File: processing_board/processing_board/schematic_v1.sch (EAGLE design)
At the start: 20 parts, among them Q1 BSS138, Q2 BSS138

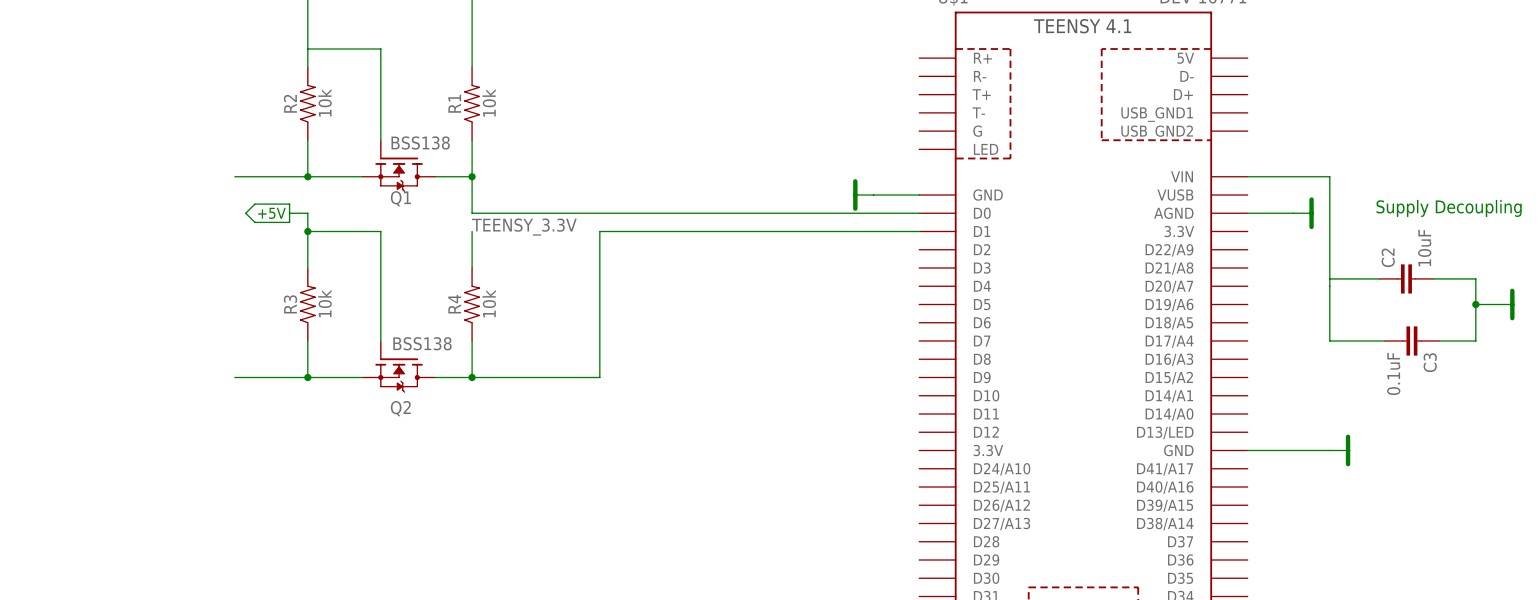
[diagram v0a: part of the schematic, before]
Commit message: modified shcematic and board
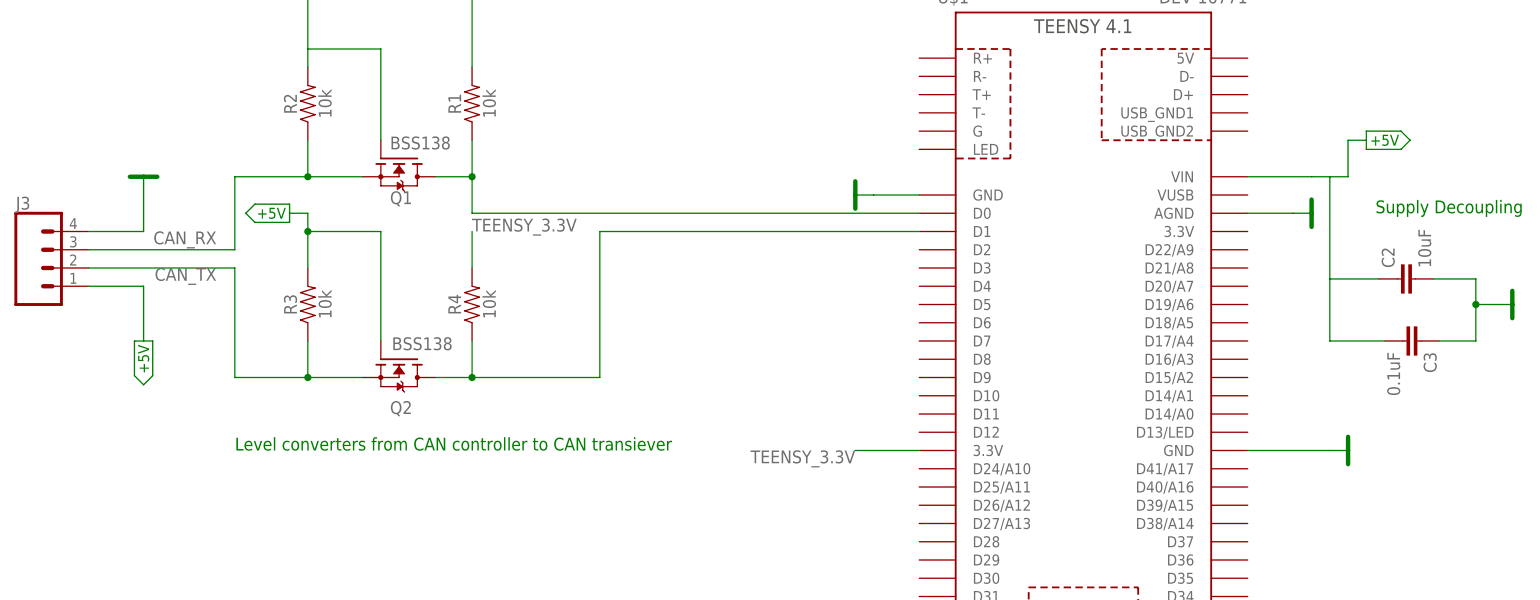
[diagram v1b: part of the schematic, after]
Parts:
- added J3: (no value), SparkFun-Connectors:CONN_04PTH
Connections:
- removed net N$11: Q2.S, R3.1
- removed net N$2: Q1.S, R2.1
- removed net VDD: C2.1, C3.2, U$1.VIN
- new net CAN_RX: J3.3, Q1.S, R2.1
- new net CAN_TX: J3.2, Q2.S, R3.1
- net +5V: now also C2.1, C3.2, J3.1, U$1.VIN
- net GND: now also J3.4
- net TEENSY_3.3V: now also U$1.3.3V
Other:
- note added: "Level converters from CAN controller to CAN transiever"
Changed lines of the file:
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@@
 <part name="PWR6" library="supply" deviceset="+5V" device=""/>
 <part name="PWR7" library="supply" deviceset="+5V" device=""/>
+<part name="PWR8" library="supply" deviceset="+5V" device=""/>
+<part name="J3" library="SparkFun-Connectors" deviceset="CONN_04" device="PTH"/>
+<part name="GND8" library="supply" deviceset="GND" device=""/>
+<part name="PWR9" library="supply" deviceset="+5V" device=""/>
 </parts>
 <sheets>
@@
 <plain>
 <text x="62.23" y="63.5" size="1.778" layer="91">Supply Decoupling</text>
+<text x="-96.52" y="30.48" size="1.778" layer="91">Level converters from CAN controller to CAN transiever</text>
 </plain>
 <instances>
@@
 <instance part="PWR6" gate="G$1" x="-86.36" y="93.98" smashed="yes"/>
 <instance part="PWR7" gate="G$1" x="-88.9" y="63.5" smashed="yes" rot="R90"/>
+<instance part="PWR8" gate="G$1" x="60.96" y="73.66" smashed="yes" rot="R270"/>
+<instance part="J3" gate="J1" x="-121.92" y="55.88" smashed="yes">
+<attribute name="VALUE" x="-127" y="48.514" size="1.778" layer="96" font="vector"/>
+<attribute name="NAME" x="-127" y="64.008" size="1.778" layer="95" font="vector"/>
+</instance>
+<instance part="GND8" gate="VR1" x="-109.22" y="68.58" smashed="yes" rot="R180"/>
+<instance part="PWR9" gate="G$1" x="-109.22" y="45.72" smashed="yes" rot="R180"/>
 </instances>
 <busses>
 </busses>
 <nets>
-<net name="VDD" class="0">
-<segment>
-<pinref part="C3" gate="G$1" pin="2"/>
-<wire x1="55.88" y1="54.356" x2="55.88" y2="53.34" width="0.1524" layer="91"/>
-<wire x1="55.88" y1="53.34" x2="55.88" y2="45.72" width="0.1524" layer="91"/>
-<wire x1="63.5" y1="45.72" x2="55.88" y2="45.72" width="0.1524" layer="91"/>
-<pinref part="C2" gate="G$1" pin="1"/>
-<wire x1="62.738" y1="54.356" x2="55.88" y2="54.356" width="0.1524" layer="91"/>
-<pinref part="U$1" gate="G$1" pin="VIN"/>
-<wire x1="44.45" y1="68.58" x2="55.88" y2="68.58" width="0.1524" layer="91"/>
-<wire x1="55.88" y1="68.58" x2="55.88" y2="54.356" width="0.1524" layer="91"/>
-</segment>
-</net>
 <net name="GND" class="0">
 <segment>
@@
 <wire x1="200.66" y1="45.72" x2="200.66" y2="48.26" width="0.1524" layer="91"/>
 </segment>
+<segment>
+<pinref part="J3" gate="J1" pin="4"/>
+<wire x1="-116.84" y1="60.96" x2="-109.22" y2="60.96" width="0.1524" layer="91"/>
+<wire x1="-109.22" y1="60.96" x2="-109.22" y2="66.04" width="0.1524" layer="91"/>
+<pinref part="GND8" gate="VR1" pin="GND"/>
+</segment>
 </net>
 <net name="+15V" class="0">
@@
 <wire x1="-88.9" y1="63.5" x2="-86.36" y2="63.5" width="0.1524" layer="91"/>
 </segment>
+<segment>
+<pinref part="PWR8" gate="G$1" pin="+5V"/>
+<wire x1="60.96" y1="73.66" x2="58.42" y2="73.66" width="0.1524" layer="91"/>
+<wire x1="58.42" y1="73.66" x2="58.42" y2="68.58" width="0.1524" layer="91"/>
+<pinref part="C3" gate="G$1" pin="2"/>
+<wire x1="55.88" y1="54.356" x2="55.88" y2="45.72" width="0.1524" layer="91"/>
+<wire x1="63.5" y1="45.72" x2="55.88" y2="45.72" width="0.1524" layer="91"/>
+<pinref part="C2" gate="G$1" pin="1"/>
+<wire x1="62.738" y1="54.356" x2="55.88" y2="54.356" width="0.1524" layer="91"/>
+<pinref part="U$1" gate="G$1" pin="VIN"/>
+<wire x1="44.45" y1="68.58" x2="53.34" y2="68.58" width="0.1524" layer="91"/>
+<wire x1="53.34" y1="68.58" x2="55.88" y2="68.58" width="0.1524" layer="91"/>
+<wire x1="55.88" y1="68.58" x2="55.88" y2="54.356" width="0.1524" layer="91"/>
+<wire x1="58.42" y1="68.58" x2="55.88" y2="68.58" width="0.1524" layer="91"/>
+</segment>
+<segment>
+<pinref part="J3" gate="J1" pin="1"/>
+<wire x1="-116.84" y1="53.34" x2="-109.22" y2="53.34" width="0.1524" layer="91"/>
+<wire x1="-109.22" y1="53.34" x2="-109.22" y2="45.72" width="0.1524" layer="91"/>
+<pinref part="PWR9" gate="G$1" pin="+5V"/>
+</segment>
 </net>
 <net name="+3.3V" class="0">
@@
 </segment>
 </net>
-<net name="N$2" class="0">
+<net name="CAN_RX" class="0">
 <segment>
 <pinref part="R2" gate="G$1" pin="1"/>
@@
 <wire x1="-86.36" y1="68.58" x2="-96.52" y2="68.58" width="0.1524" layer="91"/>
 <junction x="-86.36" y="68.58"/>
+<pinref part="J3" gate="J1" pin="3"/>
+<wire x1="-116.84" y1="58.42" x2="-96.52" y2="58.42" width="0.1524" layer="91"/>
+<wire x1="-96.52" y1="58.42" x2="-96.52" y2="68.58" width="0.1524" layer="91"/>
+<label x="-99.06" y="60.96" size="1.778" layer="95" rot="R180"/>
 </segment>
 </net>
@@
 <label x="-63.5" y="60.96" size="1.778" layer="95"/>
 </segment>
-</net>
-<net name="N$11" class="0">
+<segment>
+<pinref part="U$1" gate="G$1" pin="3.3V"/>
+<wire x1="-1.27" y1="30.48" x2="-10.16" y2="30.48" width="0.1524" layer="91"/>
+<label x="-10.16" y="30.48" size="1.778" layer="95" rot="R180"/>
+</segment>
+</net>
+<net name="CAN_TX" class="0">
 <segment>
 <pinref part="R3" gate="G$1" pin="1"/>
@@
 <wire x1="-86.36" y1="40.64" x2="-96.52" y2="40.64" width="0.1524" layer="91"/>
 <junction x="-86.36" y="40.64"/>
-</segment>
-</net>
+<wire x1="-96.52" y1="40.64" x2="-96.52" y2="55.88" width="0.1524" layer="91"/>
+<pinref part="J3" gate="J1" pin="2"/>
+<wire x1="-96.52" y1="55.88" x2="-116.84" y2="55.88" width="0.1524" layer="91"/>
+<label x="-99.06" y="55.88" size="1.778" layer="95" rot="R180"/>
+</segment>
+</net>
